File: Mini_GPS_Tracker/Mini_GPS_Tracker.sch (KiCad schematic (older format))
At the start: 19 parts, among them J1 USB_C_Receptacle, SW1 SW_Push, U1 CH340E, Y1 Crystal

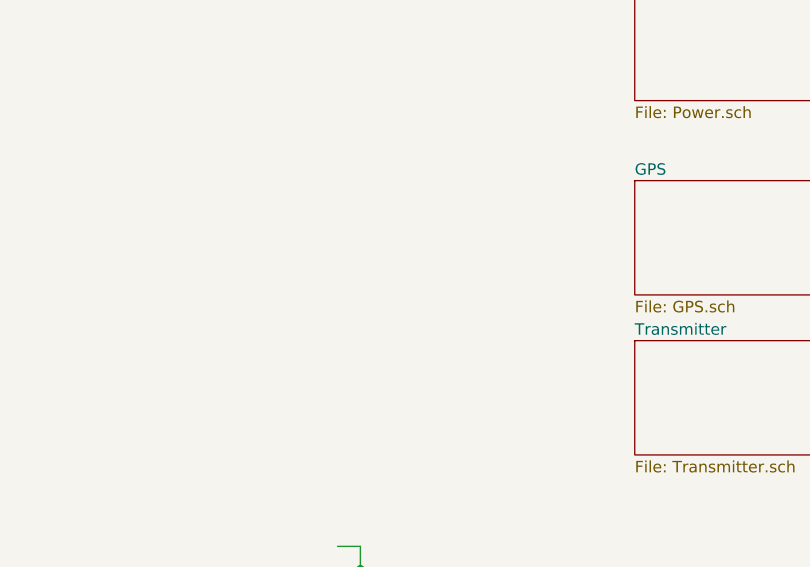
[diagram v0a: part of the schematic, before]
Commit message: updates to routing
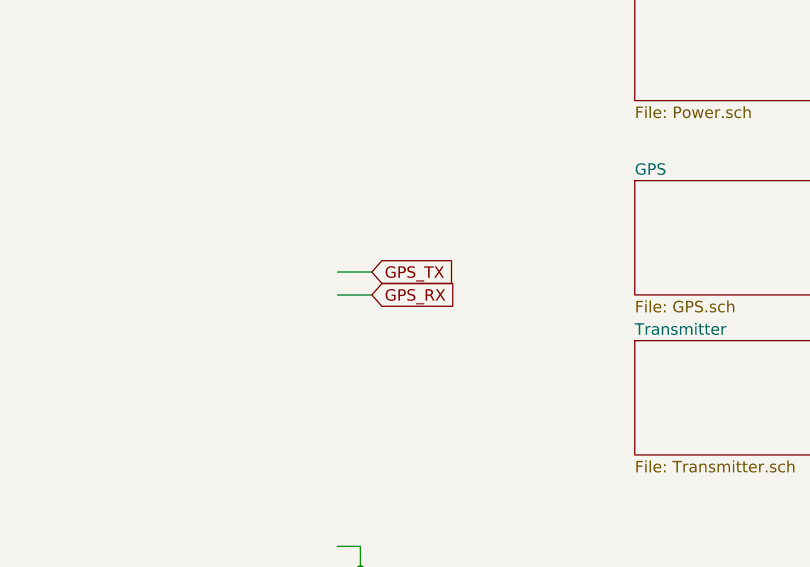
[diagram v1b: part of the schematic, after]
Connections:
- wire segments 79 -> 81
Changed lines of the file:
@@
 Wire Wire Line
 	5950 950  5950 1050
-Text GLabel 10550 4350 2    50   Input ~ 0
-GPS_TX
-Text GLabel 10550 4450 2    50   Input ~ 0
-GPS_RX
-Wire Wire Line
-	10300 4350 10550 4350
-Wire Wire Line
-	10300 4450 10550 4450
 Text GLabel 10500 5050 2    50   Input ~ 0
 TRANS_TX
@@
 Text GLabel 7650 3250 2    50   Input ~ 0
 TRANS_RX
+Wire Wire Line
+	10300 4350 10550 4350
+Wire Wire Line
+	10300 4450 10550 4450
+Text GLabel 10550 4450 2    50   Input ~ 0
+GPS_RX
+Text GLabel 10550 4350 2    50   Input ~ 0
+GPS_TX
+Text GLabel 7800 4750 2    50   Input ~ 0
+GPS_RX
+Text GLabel 7800 4650 2    50   Input ~ 0
+GPS_TX
+Wire Wire Line
+	7650 4650 7800 4650
+Wire Wire Line
+	7650 4750 7800 4750
 $EndSCHEMATC

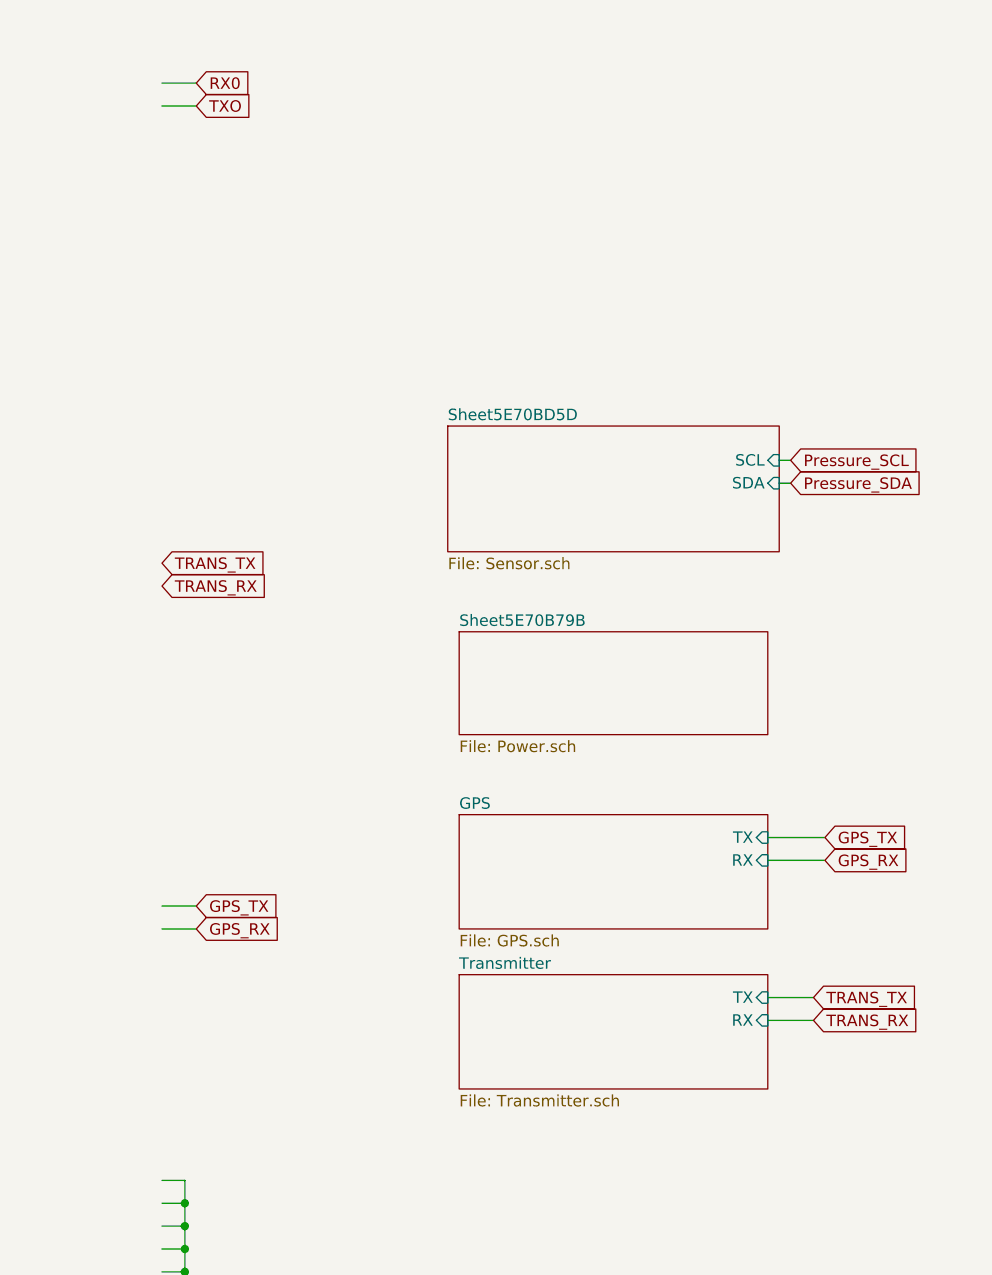
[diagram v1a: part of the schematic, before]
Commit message: worked on routing
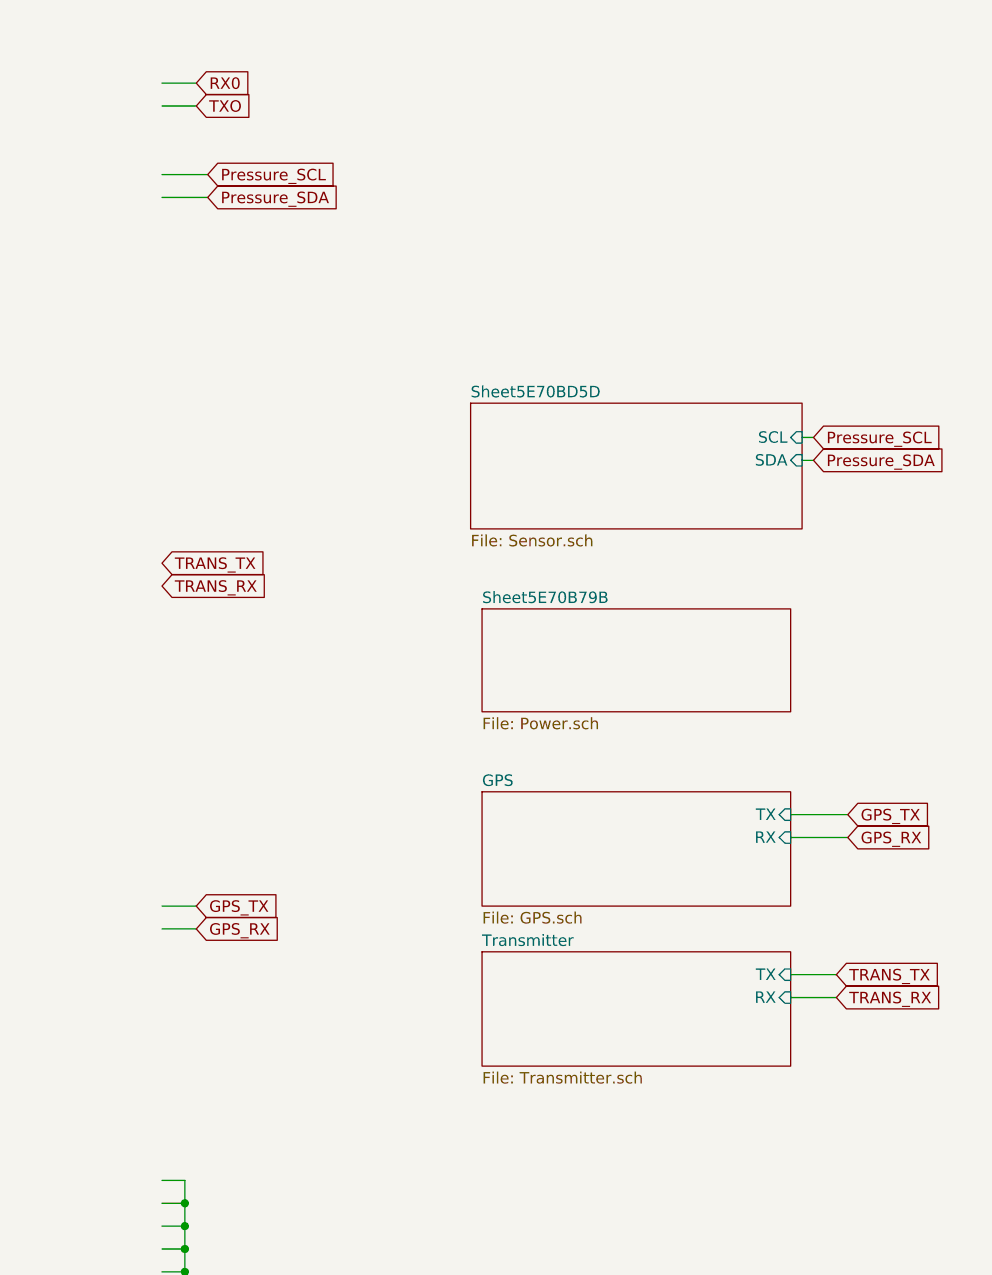
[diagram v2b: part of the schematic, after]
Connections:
- wire segments 81 -> 83
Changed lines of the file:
@@
 Comment4 ""
 $EndDescr
-$Sheet
-S 8950 4950 1350 500
-U 5E70A48E
-F0 "Transmitter" 50
-F1 "Transmitter.sch" 50
-F2 "TX" I R 10300 5050 50
-F3 "RX" I R 10300 5150 50
-$EndSheet
-$Sheet
-S 8950 4250 1350 500
-U 5E70A878
-F0 "GPS" 50
-F1 "GPS.sch" 50
-F2 "TX" I R 10300 4350 50
-F3 "RX" I R 10300 4450 50
-$EndSheet
-$Sheet
-S 8950 3450 1350 450
-U 5E70B79C
-F0 "Sheet5E70B79B" 50
-F1 "Power.sch" 50
-$EndSheet
 $Comp
 L Device:Crystal Y1
@@
 Wire Wire Line
 	5950 950  5950 1050
-Text GLabel 10500 5050 2    50   Input ~ 0
-TRANS_TX
-Text GLabel 10500 5150 2    50   Input ~ 0
-TRANS_RX
-Wire Wire Line
-	10300 5050 10500 5050
-Wire Wire Line
-	10300 5150 10500 5150
-Text GLabel 10400 2700 2    50   Input ~ 0
-Pressure_SCL
-Text GLabel 10400 2800 2    50   Input ~ 0
-Pressure_SDA
-Wire Wire Line
-	10350 2700 10400 2700
-Wire Wire Line
-	10350 2800 10400 2800
 $Comp
 L Sparkfun~Artemis:CH340E U1
@@
 Wire Wire Line
 	4450 4450 4450 4350
-$Sheet
-S 8900 2550 1450 550
-U 5E70BD5E
-F0 "Sheet5E70BD5D" 50
-F1 "Sensor.sch" 50
-F2 "SCL" I R 10350 2700 50
-F3 "SDA" I R 10350 2800 50
-$EndSheet
 $Comp
 L Sparkfun~Artemis:SPARKFUN_WRL-15376 MD1
@@
 Text GLabel 7650 3250 2    50   Input ~ 0
 TRANS_RX
-Wire Wire Line
-	10300 4350 10550 4350
-Wire Wire Line
-	10300 4450 10550 4450
-Text GLabel 10550 4450 2    50   Input ~ 0
-GPS_RX
-Text GLabel 10550 4350 2    50   Input ~ 0
-GPS_TX
 Text GLabel 7800 4750 2    50   Input ~ 0
 GPS_RX
@@
 Wire Wire Line
 	7650 4750 7800 4750
+Text GLabel 7850 1550 2    50   Input ~ 0
+Pressure_SDA
+Text GLabel 7850 1450 2    50   Input ~ 0
+Pressure_SCL
+Wire Wire Line
+	7650 1450 7850 1450
+Wire Wire Line
+	7650 1550 7850 1550
+Text GLabel 10650 4250 2    50   Input ~ 0
+GPS_TX
+Text GLabel 10650 4350 2    50   Input ~ 0
+GPS_RX
+Wire Wire Line
+	10400 4350 10650 4350
+Wire Wire Line
+	10400 4250 10650 4250
+$Sheet
+S 9000 2450 1450 550
+U 5E70BD5E
+F0 "Sheet5E70BD5D" 50
+F1 "Sensor.sch" 50
+F2 "SCL" I R 10450 2600 50
+F3 "SDA" I R 10450 2700 50
+$EndSheet
+Wire Wire Line
+	10450 2700 10500 2700
+Wire Wire Line
+	10450 2600 10500 2600
+Text GLabel 10500 2700 2    50   Input ~ 0
+Pressure_SDA
+Text GLabel 10500 2600 2    50   Input ~ 0
+Pressure_SCL
+Wire Wire Line
+	10400 5050 10600 5050
+Wire Wire Line
+	10400 4950 10600 4950
+Text GLabel 10600 5050 2    50   Input ~ 0
+TRANS_RX
+Text GLabel 10600 4950 2    50   Input ~ 0
+TRANS_TX
+$Sheet
+S 9050 3350 1350 450
+U 5E70B79C
+F0 "Sheet5E70B79B" 50
+F1 "Power.sch" 50
+$EndSheet
+$Sheet
+S 9050 4150 1350 500
+U 5E70A878
+F0 "GPS" 50
+F1 "GPS.sch" 50
+F2 "TX" I R 10400 4250 50
+F3 "RX" I R 10400 4350 50
+$EndSheet
+$Sheet
+S 9050 4850 1350 500
+U 5E70A48E
+F0 "Transmitter" 50
+F1 "Transmitter.sch" 50
+F2 "TX" I R 10400 4950 50
+F3 "RX" I R 10400 5050 50
+$EndSheet
 $EndSCHEMATC
